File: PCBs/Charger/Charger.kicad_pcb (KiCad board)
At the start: 2 copper layers, 22.5 x 19 mm, 18 parts, among them J1 Battery, J2 Charger, J3 Output 1, J4 Output 2, J5 MCU, U1 MCP73831T-2, U2 MAX17048

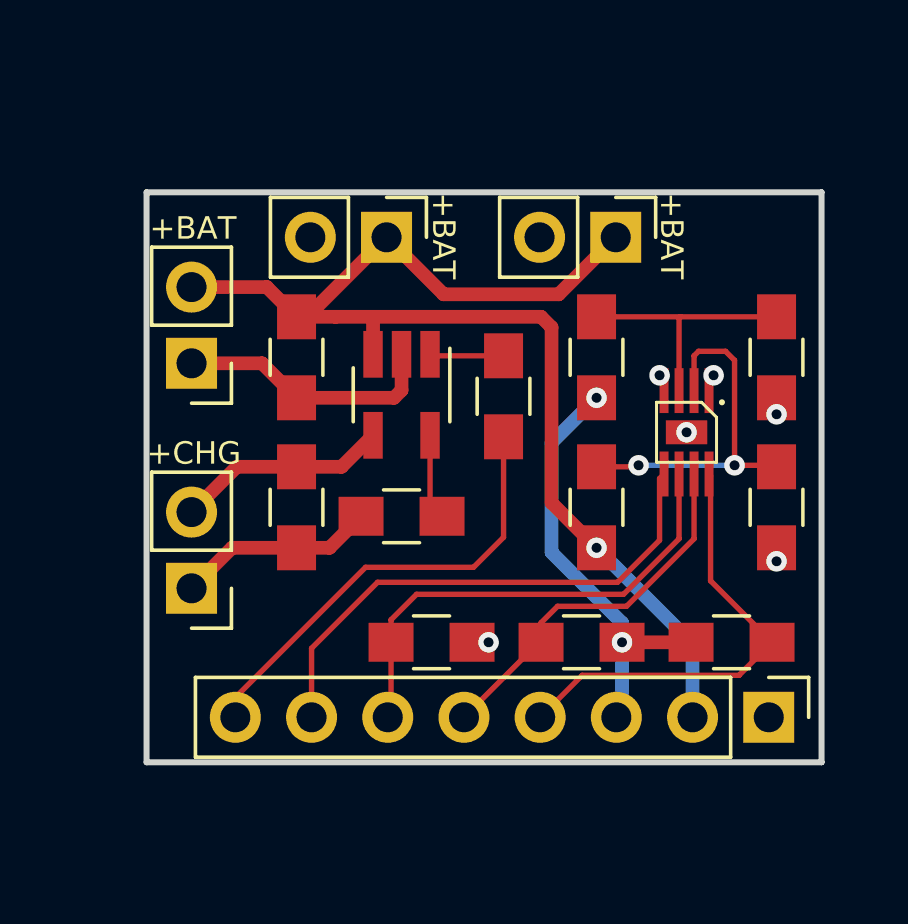
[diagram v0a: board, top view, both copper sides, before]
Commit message: Changed
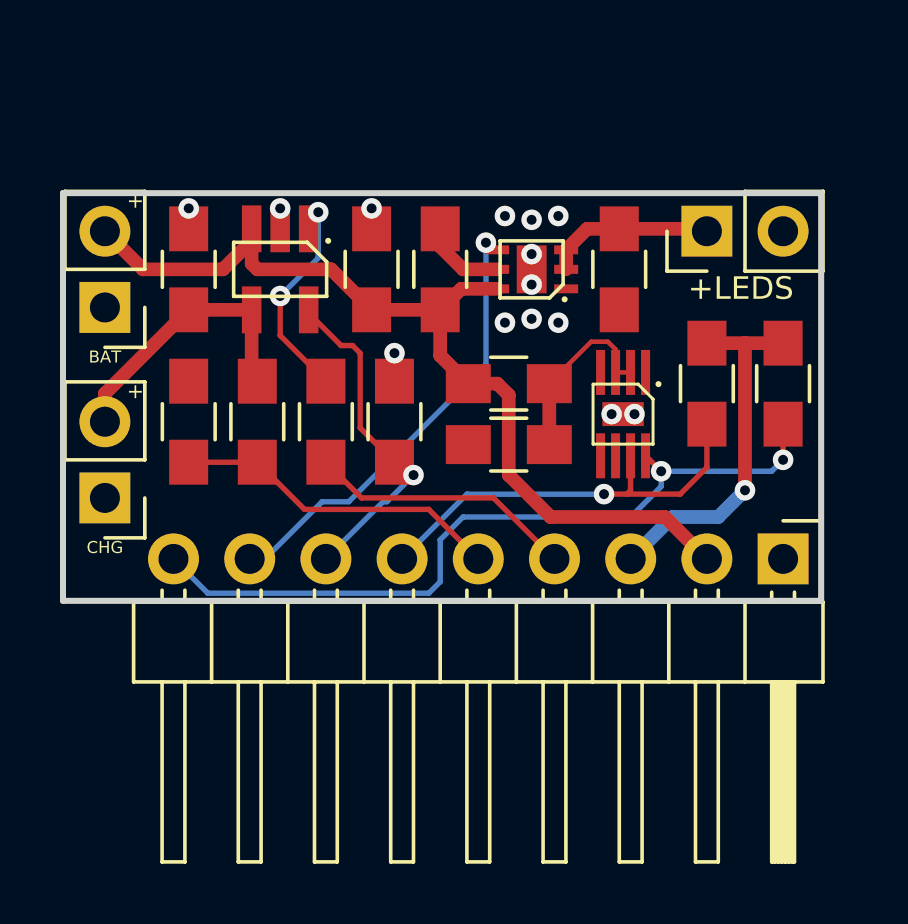
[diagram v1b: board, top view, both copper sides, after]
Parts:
- removed J5: MCU, Pin_Headers:Pin_Header_Straight_1x08_Pitch2.54mm
- added L1: 1uH, Inductors_SMD:L_0805_HandSoldering, F.Cu at (145.3, 99.6)
- added U3: MAX17048, my-smd:TDFN-T822+1, F.Cu at (151.4, 104.4)
- C3: value 1uF -> 10uF
- C4: value 10nF -> 1uF
- J3: value Output 1 -> LEDs
- J4: value Output 2 -> MCU; footprint Pin_Headers:Pin_Header_Straight_1x02_Pitch2.54mm -> Pin_Headers:Pin_Header_Angled_1x09_Pitch2.54mm
- R2: value 1K -> 2K
- R3: value 1K -> 2.2K
- R4: value 150 -> 3.3K
- R5: value 4.7K -> 1K
- U1: footprint TO_SOT_Packages_SMD:SOT-23-5_HandSoldering -> my-smd:SOT-23-5_HandSoldering
- U2: value MAX17048 -> TPS61240; footprint my-smd:TDFN-T822+1 -> my-smd:WSON6_2.1x2.1mm_Pitch0.65mm
- moved R4 13.8 mm to (136.9, 104.6)
- moved R7 12.6 mm to (154.2, 103.4), turned to 270 degrees
- moved J4 12.1 mm to (156.7, 109.2)
- moved R5 11.4 mm to (147.6, 103.4)
- moved R6 10.9 mm to (156.7, 103.4), turned to 270 degrees
- moved J3 10.7 mm to (154.2, 98.3), turned to 90 degrees
- moved C3 9.51 mm to (151.3, 99.6)
- moved C4 9.39 mm to (147.6, 105.4), turned to 180 degrees
- moved C1 8.71 mm to (136.9, 99.6), turned to 90 degrees
- moved R3 8.25 mm to (139.2, 104.6), turned to 270 degrees
- moved U2 7.49 mm to (148.3, 99.6), turned to 180 degrees
- moved R2 7.31 mm to (143.8, 104.6), turned to 90 degrees
- moved U1 5.82 mm to (140.0, 99.6)
- moved J2 4.17 mm to (134.1, 107.2)
- moved R1 4.04 mm to (141.5, 104.6), turned to 90 degrees
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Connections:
- C3 pad 1: Net-(C3-Pad1) -> /VLED
- C4 pad 1: Net-(C4-Pad1) -> /CELL
- J3 pad 1: /VBAT -> /VLED
- J4 pad 1: /VBAT -> GND
- J4 pad 2: GND -> /VBAT
- R1 pad 1: Net-(R1-Pad1) -> /~CHARGING
- R1 pad 2: GND -> /STAT
- R2 pad 1: Net-(C3-Pad1) -> /~CHG_EN
- R2 pad 2: /VBAT -> GND
- R3 pad 1: /~STAT -> /VCHG
- R3 pad 2: Net-(R3-Pad2) -> /CHG_PRESENT
- R4 pad 1: /3.3V -> /CHG_PRESENT
- R4 pad 2: Net-(C4-Pad1) -> GND
- R5 pad 1: /3.3V -> /VBAT
- R5 pad 2: /SDA -> /CELL
- R6 pad 2: /SCL -> /SDA
- R7 pad 1: /QSTRT -> /3.3V
- R7 pad 2: GND -> /SCL
- U1 pad 1: Net-(R3-Pad2) -> /STAT
- U1 pad 5: Net-(R1-Pad1) -> /~CHG_EN
- U2 pad 2: Net-(C3-Pad1) -> /VLED
- U2 pad 3: Net-(C4-Pad1) -> /VLED
- U2 pad 4: GND -> /LED_EN
- U2 pad 5: /~ALRT -> /L
- U2 pad 6: /QSTRT -> /VBAT
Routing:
- net /~ALRT: track 17.7 -> 0.00 mm
- net /QSTRT: track 16.2 -> 0.00 mm
- net GND: track 15.8 -> 0.00 mm, vias 6 -> 14
- net /~STAT: track 15.2 -> 0.00 mm
- net /LED_EN: track 0.00 -> 15.1 mm, vias 0 -> 1
- net Net-(C3-Pad1): track 12.4 -> 0.00 mm, vias 2 -> 0
- net /~CHG_EN: track 0.00 -> 11.4 mm, vias 0 -> 1
- net /CHG_PRESENT: track 0.00 -> 11.0 mm
- net /VBAT: track 42.1 -> 31.3 mm, vias 1 -> 0
- net /SDA: track 15.2 -> 25.7 mm, vias 0 -> 2
- net /~CHARGING: track 0.00 -> 8.95 mm
- net Net-(C4-Pad1): track 8.48 -> 0.00 mm
- net /STAT: track 0.00 -> 7.48 mm, vias 0 -> 2
- net /CELL: track 0.00 -> 6.19 mm
- net /VLED: track 0.00 -> 5.67 mm
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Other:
- board size 22.5 x 19 mm -> 25.3 x 13.6 mm
- rule solder_mask_min_width: 0.101 -> 0.1016
- board text added: "+"
- board text added: "+LEDS"
- board text added: "BAT"
- board text added: "CHG"
- board text added: "CHG_PRESENT"
- board text added: "LED_EN"
- board text added: "Power Supply v1"
- board text added: "~CHARGING"
- board text added: "~CHG_EN"
- board text removed: "+BAT"
- board text removed: "+CHG"
- board text removed: "Charger v1"
- board text removed: "QSTRT"
- board text removed: "~ALRT"
- board text removed: "~STAT"

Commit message: New design and layout
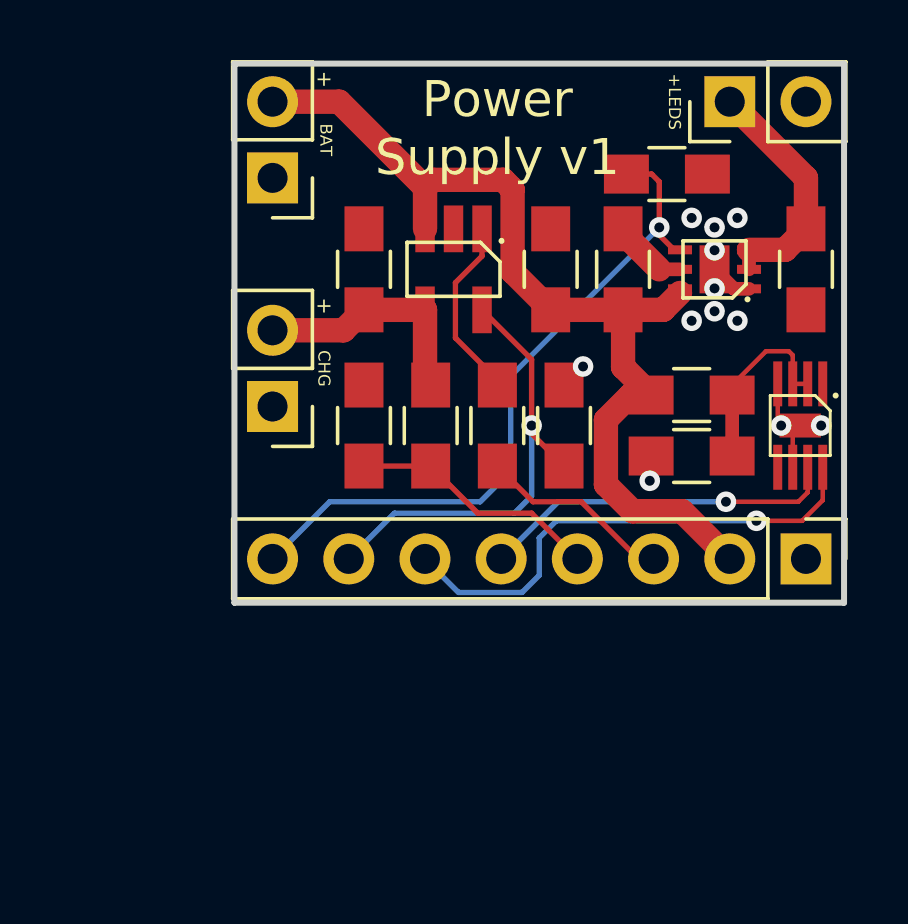
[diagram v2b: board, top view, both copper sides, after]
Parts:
- removed R7: 4.7K, Resistors_SMD:R_0805_HandSoldering
- J4: footprint Pin_Headers:Pin_Header_Angled_1x09_Pitch2.54mm -> Pin_Headers:Pin_Header_Straight_1x08_Pitch2.54mm
- R5: value 1K -> 10K
- R6: value 4.7K -> 1K
- moved R5 8.75 mm to (152.8, 96.4)
- moved J1 7.06 mm to (139.7, 96.5)
- moved J2 6.37 mm to (139.7, 104.1)
- moved C3 6.22 mm to (157.5, 99.6)
- moved C4 6.11 mm to (153.7, 105.8)
- moved L1 6.10 mm to (151.4, 99.6)
- moved U2 6.10 mm to (154.4, 99.6)
- moved C2 5.97 mm to (149.0, 99.6)
- moved U3 5.92 mm to (157.3, 104.8)
- moved R4 5.84 mm to (142.7, 104.8)
- moved C1 5.84 mm to (142.7, 99.6)
- moved R3 5.78 mm to (145.0, 104.8)
- moved U1 5.78 mm to (145.7, 99.6)
- moved R1 5.72 mm to (147.2, 104.8)
- moved R2 5.65 mm to (149.4, 104.8)
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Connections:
- J4 pad 3: /3.3V -> /~CHARGING
- J4 pad 4: /~CHARGING -> /CHG_PRESENT
- J4 pad 5: /CHG_PRESENT -> /SCL
- J4 pad 6: /SCL -> /SDA
- R5 pad 1: /VBAT -> /LED_EN
- R5 pad 2: /CELL -> GND
- R6 pad 1: /3.3V -> /VBAT
- R6 pad 2: /SDA -> /CELL
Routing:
- net /3.3V: track 12.2 -> 0.00 mm, vias 1 -> 0
- net /SDA: track 25.7 -> 16.8 mm, vias 2 -> 1
- net /LED_EN: track 15.1 -> 23.7 mm
- net GND: track 0.00 -> 4.35 mm, vias 14 -> 12
- net /~CHG_EN: track 11.4 -> 15.7 mm
- net /VLED: track 5.67 -> 8.70 mm
- net /CHG_PRESENT: track 11.0 -> 8.39 mm
- net /~CHARGING: track 8.95 -> 6.49 mm
- net /SCL: track 14.2 -> 12.0 mm
- net /VBAT: track 31.3 -> 32.5 mm
- net /STAT: track 7.48 -> 6.30 mm, vias 2 -> 0
- net /VCHG: track 9.44 -> 8.29 mm
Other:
- board size 25.3 x 13.6 mm -> 20.3 x 18 mm
- net class Big Power added: clearance 0.1524, trace_width 0.8128, via_dia 0.6858, via_drill 0.3302
- board text removed: "3.3V"
